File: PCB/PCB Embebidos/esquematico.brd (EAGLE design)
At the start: 90.9 x 66.4 mm, 34 parts, among them IC1 LM358N, IC2 317T, T1 BT138-V, T2 BT138-V

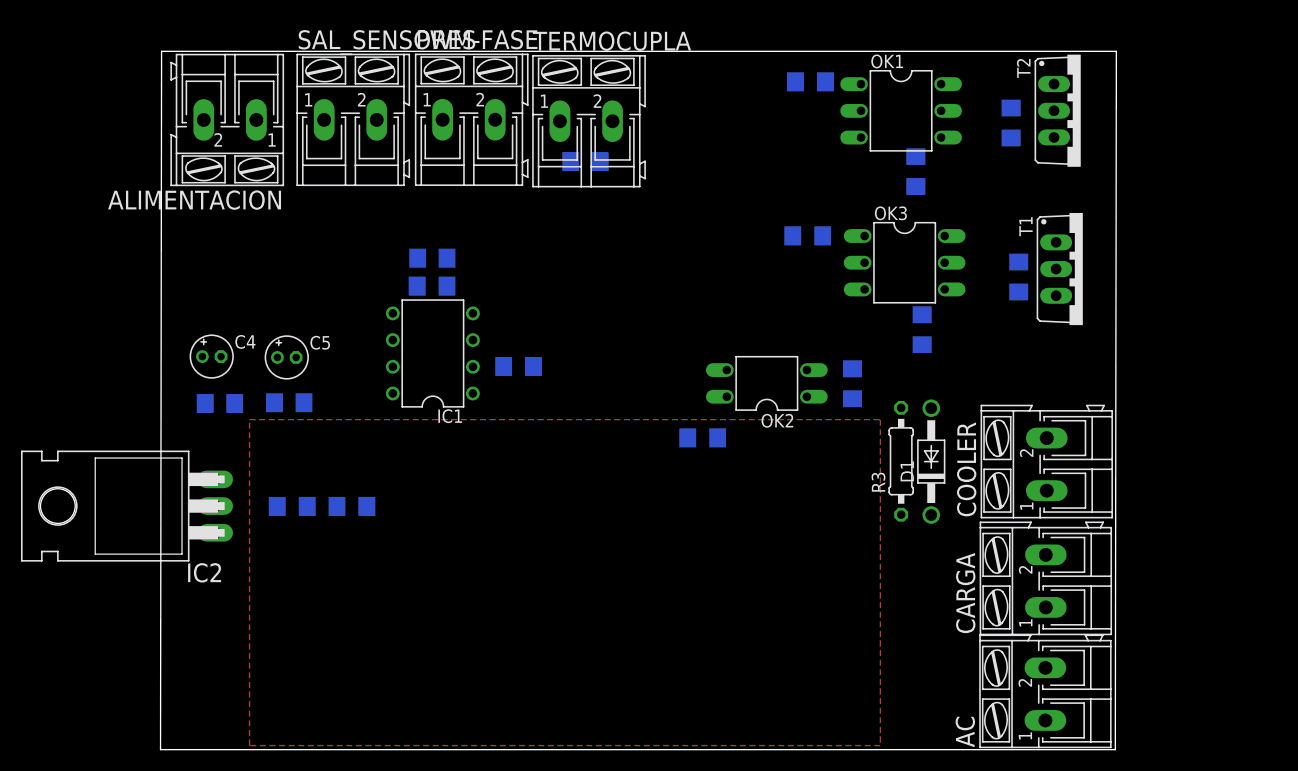
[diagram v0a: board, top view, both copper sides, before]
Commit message: El PCB esta listo para ser imprimido. Voy a comprar todos los componentes mañana y ya lo termino
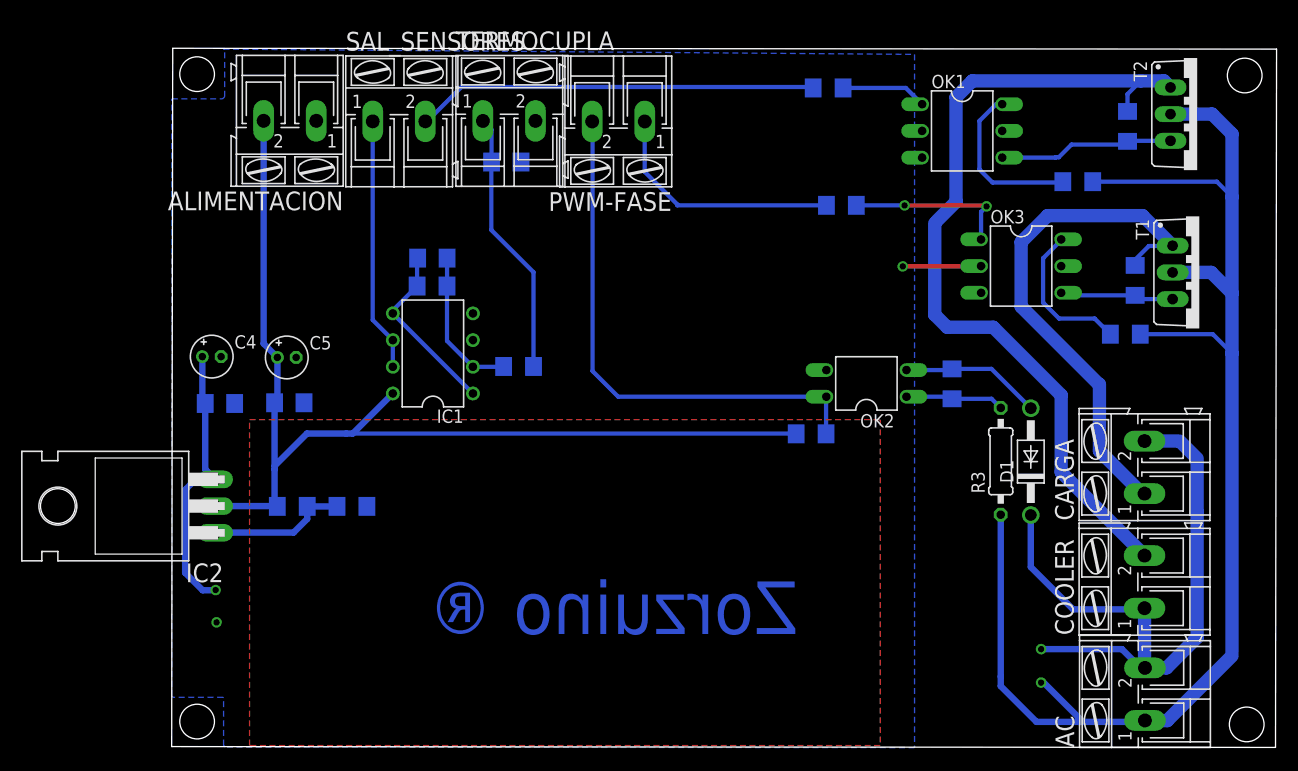
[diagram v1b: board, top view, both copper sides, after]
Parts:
- moved R1 19.3 mm to (91.8, 39.5), turned to 180 degrees
- moved R12 15.4 mm to (87.3, 54.0), turned to 180 degrees
- moved COOLER 14.5 mm to (93.6, 16.0)
- moved CARGA 14.3 mm to (93.6, 26.9)
- moved PWM-FASE 14.2 mm to (43.5, 59.8), turned to 180 degrees
- moved OK3 11.1 mm to (81.9, 46.0)
- moved R13 11.1 mm to (92.0, 59.3)
- moved R2 11.1 mm to (92.7, 44.6)
- moved T1 11.1 mm to (98.8, 45.4)
- moved T2 11.1 mm to (98.6, 60.5)
- moved R5 10.3 mm to (61.9, 30.0)
- moved D1 9.47 mm to (82.8, 27.4)
- moved R3 9.47 mm to (79.9, 27.4)
- moved OK2 9.47 mm to (67.2, 34.8)
- moved AC 9.47 mm to (93.7, 5.29)
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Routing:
- net AC+: track 0.00 -> 134.3 mm, vias 0 -> 1
- net VCC: track 0.00 -> 101.5 mm
- net N$17: track 0.00 -> 80.1 mm
- net AC-: track 0.00 -> 63.0 mm, vias 0 -> 1
- net FASE: track 0.00 -> 51.2 mm
- net N$4: track 0.00 -> 50.3 mm
- net COOLER_PIN: track 0.00 -> 38.5 mm
- net VCC_5V: track 0.00 -> 27.0 mm, vias 0 -> 1
- net TERMOCUPLA: track 0.00 -> 25.4 mm
- net SAL_TERMOCUPLA: track 0.00 -> 24.1 mm
- net PWM: track 0.00 -> 23.6 mm
- net N$15: track 0.00 -> 17.3 mm
- net N$7: track 0.00 -> 17.0 mm
- net N$12: track 0.00 -> 16.1 mm
- net N$1: track 0.00 -> 15.8 mm, vias 0 -> 2
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- added copper zone on layer 16, net GND
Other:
- board size 90.9 x 66.4 mm -> 105.1 x 66.5 mm
- board text added: "Zorzuino ®"
